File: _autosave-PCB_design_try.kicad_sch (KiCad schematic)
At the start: 22 parts

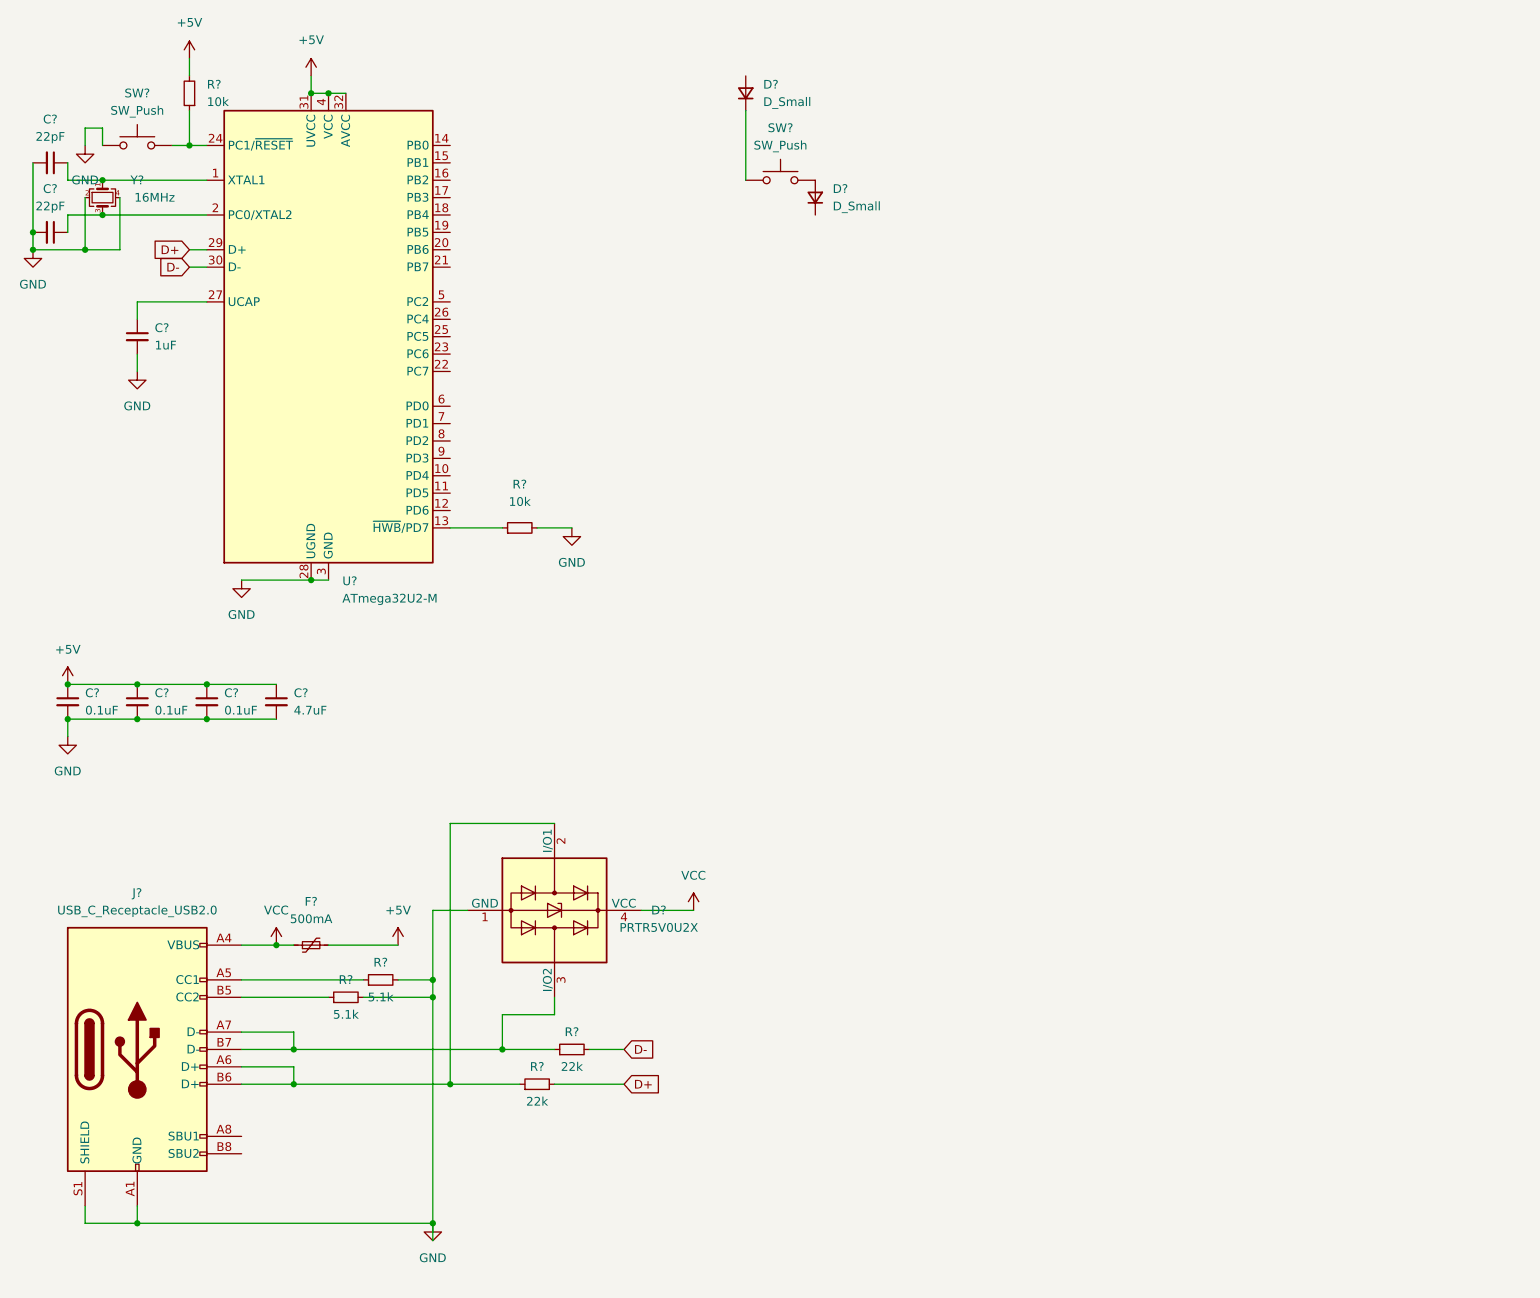
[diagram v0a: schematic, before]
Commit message: scm_finished
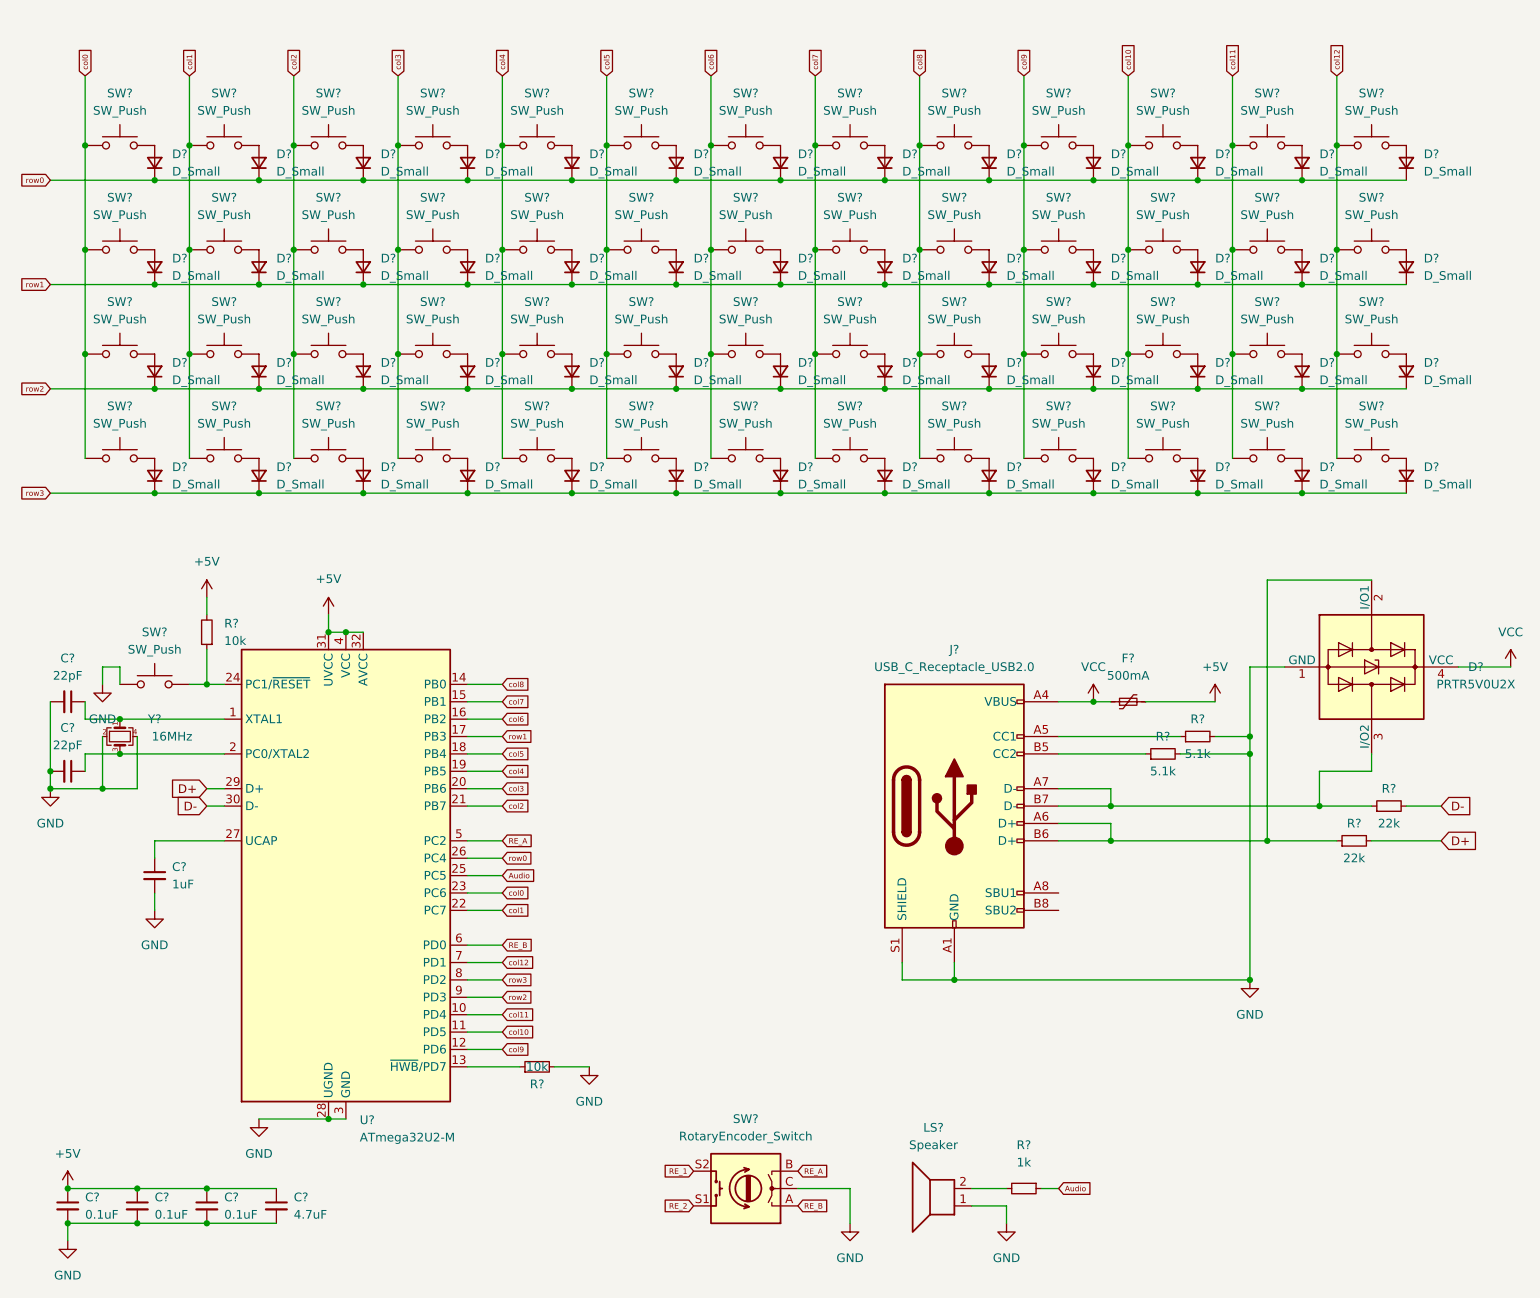
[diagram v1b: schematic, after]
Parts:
- removed D?: D_Small, symbol Device:D_Small
- added D? (x51): D_Small, symbol Device:D_Small
- added LS?: Speaker, symbol Device:Speaker
- added R?: 1k, symbol Device:R_Small
- added SW? (x51): SW_Push, symbol Switch:SW_Push
- added SW?: RotaryEncoder_Switch, symbol Device:RotaryEncoder_Switch
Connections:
- net GND: now also LS?.1, SW?.C
- net col0: now reaches SW?.1
- net col0: now also U?.23 (PC6), SW?.1, SW?.1, SW?.1
- net row0: now reaches D?.1 (K)
- net row0: now also U?.26 (PC4), D?.1 (K), D?.1 (K), D?.1 (K), D?.1 (K), D?.1 (K), D?.1 (K), D?.1 (K), D?.1 (K), D?.1 (K), D?.1 (K), D?.1 (K), D?.1 (K)
- net col11: now reaches U?.10 (PD4)
- net col11: now also SW?.1, SW?.1, SW?.1, SW?.1
- net col10: now reaches U?.11 (PD5)
- net col10: now also SW?.1, SW?.1, SW?.1, SW?.1
- net col9: now reaches U?.12 (PD6)
- net col9: now also SW?.1, SW?.1, SW?.1, SW?.1
- net col8: now reaches U?.14 (PB0)
- net col8: now also SW?.1, SW?.1, SW?.1, SW?.1
- net col7: now reaches U?.15 (PB1)
- net col7: now also SW?.1, SW?.1, SW?.1, SW?.1
- net col6: now reaches U?.16 (PB2)
- net col6: now also SW?.1, SW?.1, SW?.1, SW?.1
- net row1: now reaches U?.17 (PB3)
- net row1: now also D?.1 (K), D?.1 (K), D?.1 (K), D?.1 (K), D?.1 (K), D?.1 (K), D?.1 (K), D?.1 (K), D?.1 (K), D?.1 (K), D?.1 (K), D?.1 (K), D?.1 (K)
- net col5: now reaches U?.18 (PB4)
- net col5: now also SW?.1, SW?.1, SW?.1, SW?.1
- net col4: now reaches U?.19 (PB5)
- net col4: now also SW?.1, SW?.1, SW?.1, SW?.1
- net col3: now reaches U?.20 (PB6)
- net col3: now also SW?.1, SW?.1, SW?.1, SW?.1
- net col2: now reaches U?.21 (PB7)
- net col2: now also SW?.1, SW?.1, SW?.1, SW?.1
- net col1: now reaches U?.22 (PC7)
- net col1: now also SW?.1, SW?.1, SW?.1, SW?.1
- net Audio: now reaches U?.25 (PC5)
- net Audio: now also R?.1
- net RE_A: now reaches U?.5 (PC2)
- net RE_A: now also SW?.B
- net RE_B: now reaches U?.6 (PD0)
- net RE_B: now also SW?.A
- net col12: now reaches U?.7 (PD1)
- net col12: now also SW?.1, SW?.1, SW?.1, SW?.1
- net row3: now reaches U?.8 (PD2)
- net row3: now also D?.1 (K), D?.1 (K), D?.1 (K), D?.1 (K), D?.1 (K), D?.1 (K), D?.1 (K), D?.1 (K), D?.1 (K), D?.1 (K), D?.1 (K), D?.1 (K), D?.1 (K)
- net row2: now reaches U?.9 (PD3)
- net row2: now also D?.1 (K), D?.1 (K), D?.1 (K), D?.1 (K), D?.1 (K), D?.1 (K), D?.1 (K), D?.1 (K), D?.1 (K), D?.1 (K), D?.1 (K), D?.1 (K), D?.1 (K)
- new net: D?.2 (A), SW?.2 (x51)
- new net: LS?.2, R?.2
- new net RE_1: SW?.S2
- new net RE_2: SW?.S1
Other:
- moved on the sheet: C?, D?, F?, J?, R?, SW?, U?, Y?
